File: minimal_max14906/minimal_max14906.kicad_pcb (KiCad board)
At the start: 4 copper layers, 34.3 x 21.6 mm, 56 parts, among them Q1 SI7309DN-T1-E3, Q2 SI7309DN-T1-E3, Q3 SI7309DN-T1-E3, Q4 SI7309DN-T1-E3, U1 MAX14906ATM+

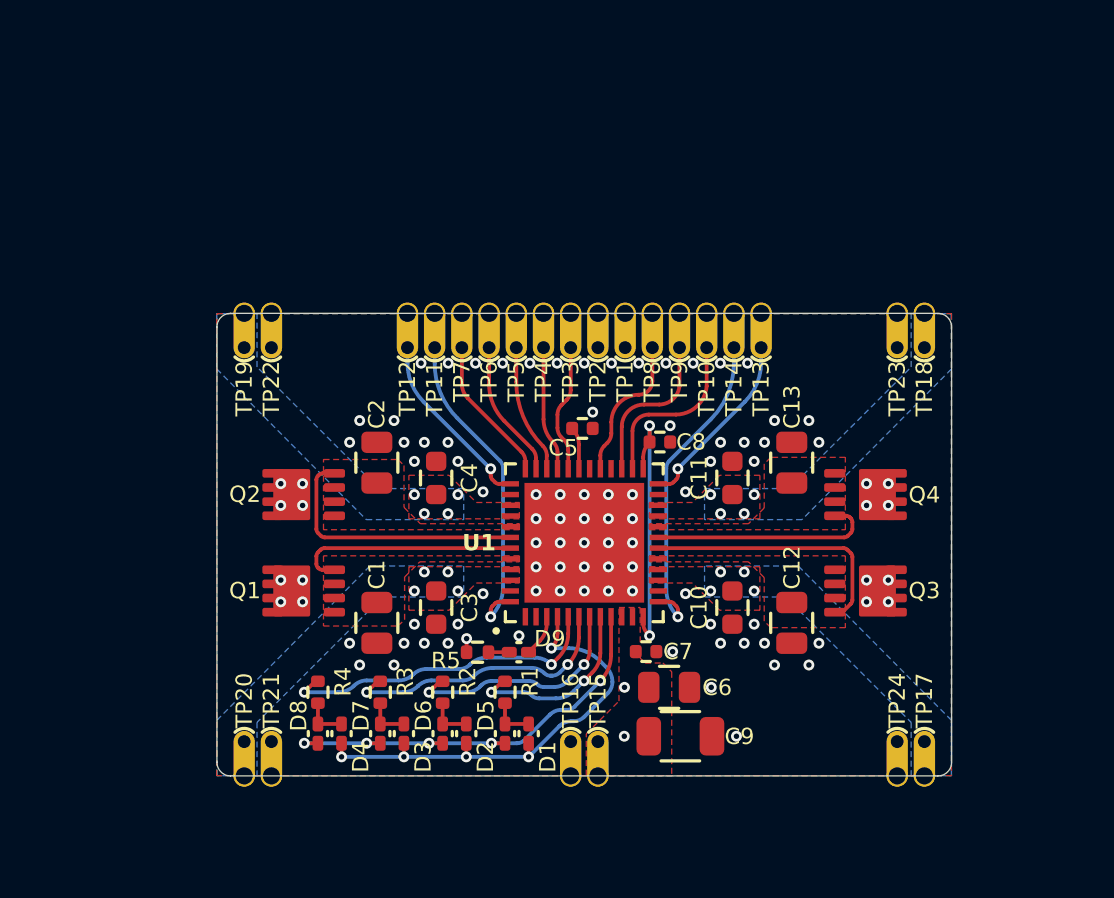
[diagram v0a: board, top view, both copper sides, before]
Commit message: Minor updates
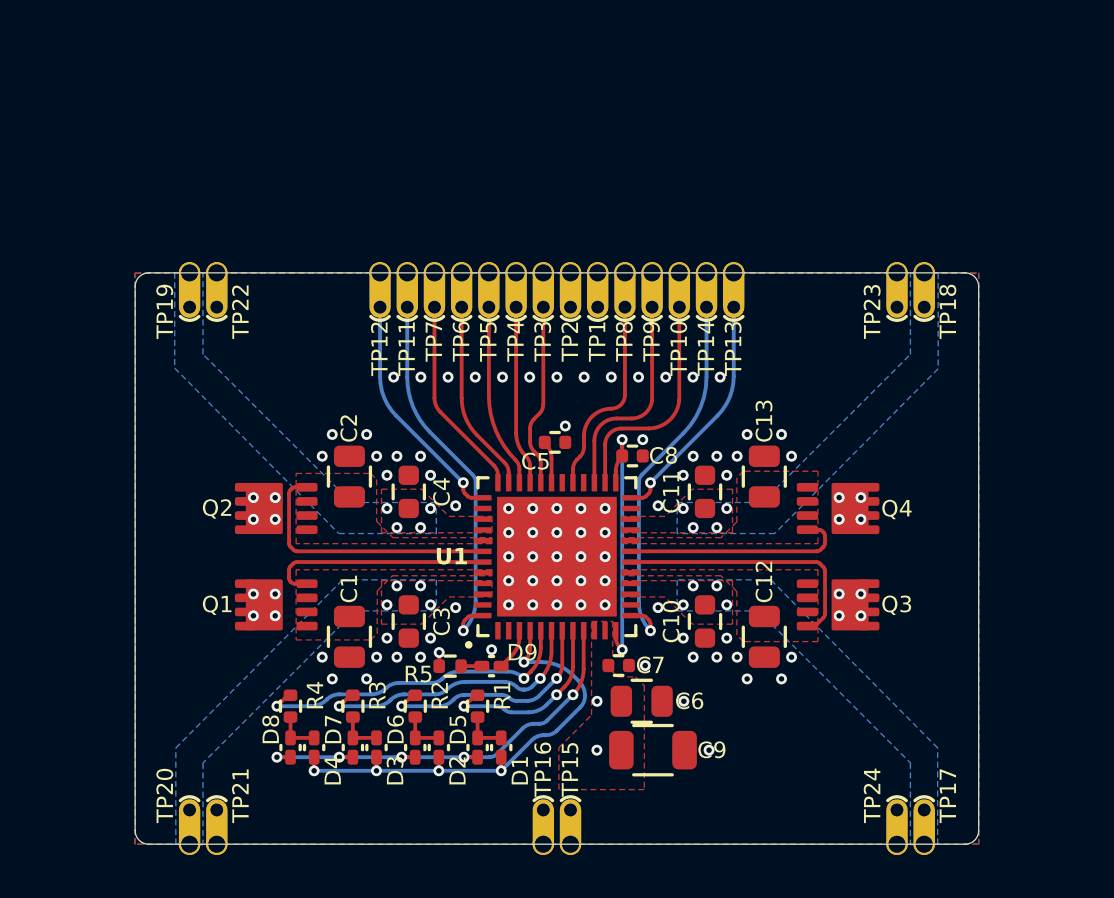
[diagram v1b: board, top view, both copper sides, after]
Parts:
- moved TP20 4.08 mm to (118.1, 116.8)
- moved TP21 4.08 mm to (119.4, 116.8)
- moved TP15 3.44 mm to (135.9, 116.8)
- moved TP16 3.44 mm to (134.6, 116.8)
- moved TP17 3.19 mm to (152.4, 116.8)
- moved TP24 3.19 mm to (151.1, 116.8)
- moved TP19 3.17 mm to (118.1, 90.2)
- moved TP22 3.17 mm to (119.4, 90.2)
- moved TP2 2.28 mm to (135.9, 90.2)
- moved TP7 2.28 mm to (129.5, 90.2)
- moved TP1 2.28 mm to (137.2, 90.2)
- moved TP10 2.28 mm to (141.0, 90.2)
- moved TP11 2.28 mm to (128.3, 90.2)
- moved TP12 2.28 mm to (127.0, 90.2)
- moved TP13 2.28 mm to (143.5, 90.2)
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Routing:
- net /D2_ISO: track 8.57 -> 11.1 mm
- net /D3_ISO: track 8.58 -> 11.1 mm
- net /D4_ISO: track 15.3 -> 17.8 mm
- net /D1_ISO: track 15.2 -> 17.8 mm
- net /MAX14906_EN_ISO: track 7.43 -> 9.97 mm
- net /MAX14906_SYNCH_ISO: track 6.81 -> 9.35 mm
- net /MAX14906_READY_ISO: track 8.10 -> 10.6 mm
- net /SPI1_SCK_ISO: track 5.82 -> 8.36 mm
- net /SPI1_MOSI_ISO: track 6.42 -> 8.96 mm
- net /SPI1_MISO_ISO: track 6.00 -> 8.54 mm
- net /SPI1_SS3_ISO: track 6.01 -> 8.55 mm
- net /MAX14906_FAULT_ISO: track 6.82 -> 9.36 mm
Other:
- board size 34.3 x 21.6 mm -> 39.4 x 26.7 mm

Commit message: Minor updates
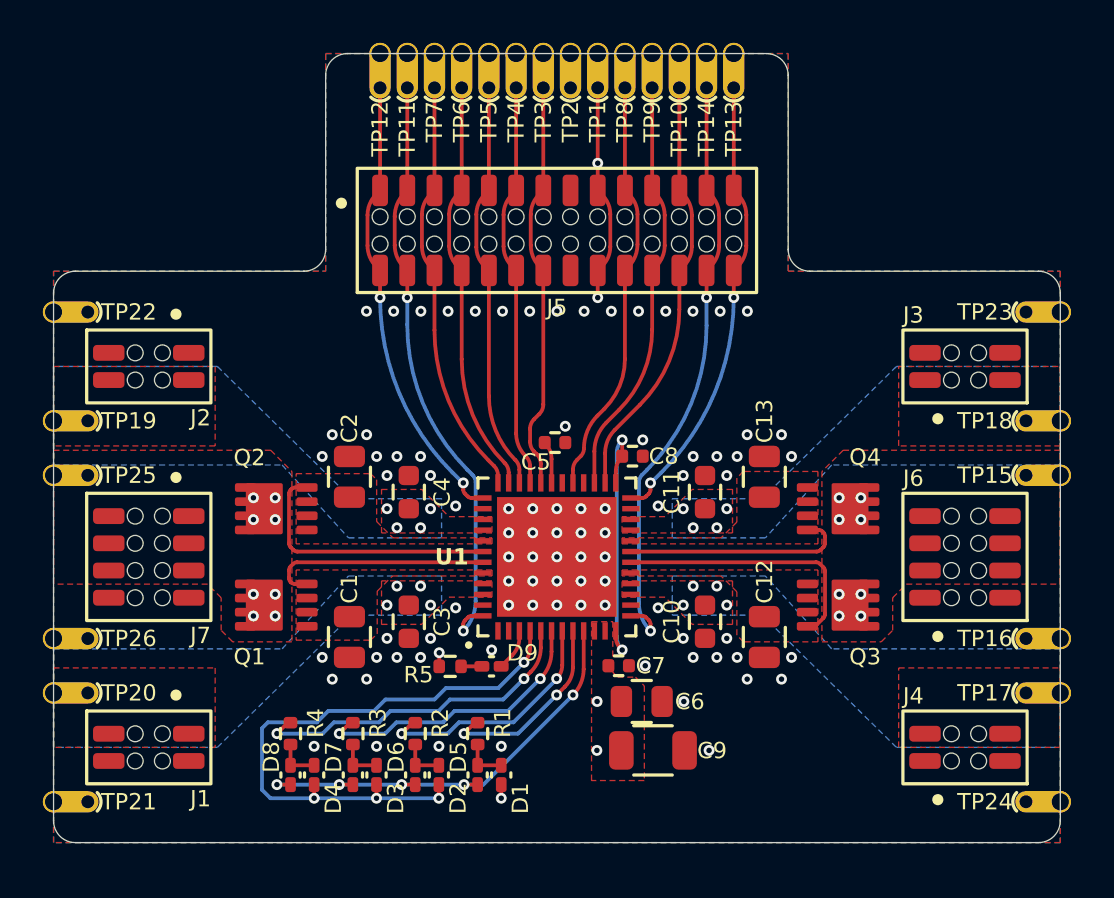
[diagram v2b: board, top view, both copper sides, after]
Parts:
- added J1: CLP-102-02-G-D-BE, connector_footprints:CLP-102-02-G-D-BE, F.Cu at (116.2, 112.3)
- added J2: CLP-102-02-G-D-BE, connector_footprints:CLP-102-02-G-D-BE, F.Cu at (116.2, 94.5)
- added J3: CLP-102-02-G-D-BE, connector_footprints:CLP-102-02-G-D-BE, F.Cu at (154.3, 94.5)
- added J4: CLP-102-02-G-D-BE, connector_footprints:CLP-102-02-G-D-BE, F.Cu at (154.3, 112.3)
- added J5: CLP-114-02-G-D-BE, connector_footprints:CLP-114-02-G-D-BE, F.Cu at (135.3, 88.2)
- added J6: CLP-104-02-G-D-BE, connector_footprints:CLP-104-02-G-D-BE, F.Cu at (154.3, 103.4)
- added J7: CLP-104-02-G-D-BE, connector_footprints:CLP-104-02-G-D-BE, F.Cu at (116.2, 103.4)
- added TP25: TestPoint, test_point_footprints:TestPoint_THTPad_Castelated, F.Cu at (111.8, 99.6)
- added TP26: TestPoint, test_point_footprints:TestPoint_THTPad_Castelated, F.Cu at (111.8, 107.2)
- moved TP15 28.6 mm to (158.7, 99.6), turned to 180 degrees
- moved TP16 26.0 mm to (158.7, 107.2), turned to 180 degrees
- moved TP1 10.2 mm to (137.2, 79.9)
- moved TP10 10.2 mm to (141.0, 79.9)
- moved TP11 10.2 mm to (128.3, 79.9)
- moved TP12 10.2 mm to (127.0, 79.9)
- moved TP13 10.2 mm to (143.5, 79.9)
- moved TP14 10.2 mm to (142.2, 79.9)
- moved TP2 10.2 mm to (135.9, 79.9)
- moved TP3 10.2 mm to (134.6, 79.9)
- moved TP4 10.2 mm to (133.4, 79.9)
- moved TP5 10.2 mm to (132.1, 79.9)
- moved TP6 10.2 mm to (130.8, 79.9)
- moved TP7 10.2 mm to (129.5, 79.9)
- moved TP8 10.2 mm to (138.4, 79.9)
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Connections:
- net /3V3_ISO renamed /3V3
- net /D1_ISO renamed /D1
- net /D2_ISO renamed /D2
- net /D3_ISO renamed /D3
- net /D4_ISO renamed /D4
- net /MAX14906_EN_ISO renamed /EN
- net /MAX14906_FAULT_ISO renamed /~{FAULT}
- net /MAX14906_READY_ISO renamed /~{READY}
- net /MAX14906_SYNCH_ISO renamed /SYNCH
- net /SPI1_MISO_ISO renamed /SDO
- net /SPI1_MOSI_ISO renamed /SDI
- net /SPI1_SCK_ISO renamed /CLK
- net /SPI1_SS3_ISO renamed /~{CS}
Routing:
- net /~{CS}: track 8.55 -> 19.2 mm
- net /CLK: track 8.36 -> 19.0 mm
- net /SDO: track 8.54 -> 19.1 mm
- net /SDI: track 8.96 -> 19.4 mm
- net /D1: track 17.8 -> 28.1 mm, vias 1 -> 2
- net /D4: track 17.8 -> 28.1 mm, vias 1 -> 2
- net /SYNCH: track 9.35 -> 19.6 mm
- net /D2: track 11.1 -> 21.3 mm, vias 1 -> 2
- net /D3: track 11.1 -> 21.3 mm, vias 1 -> 2
- net /3V3: track 13.0 -> 23.2 mm, vias 2 -> 4
- net /~{FAULT}: track 9.36 -> 19.5 mm
- net /EN: track 9.97 -> 19.6 mm
- net /~{READY}: track 10.6 -> 19.9 mm
- net /FLED: track 21.8 -> 28.9 mm
- net /SLED: track 20.6 -> 21.2 mm
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- added copper zone on In1.Cu, net /CHANNEL_1
- added copper zone on In1.Cu, net /CHANNEL_2
- added copper zone on In1.Cu, net /CHANNEL_3
- added copper zone on In1.Cu, net /CHANNEL_4
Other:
- board size 39.4 x 26.7 mm -> 47 x 36.8 mm
